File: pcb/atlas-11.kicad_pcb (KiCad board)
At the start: 2 copper layers, 115.2 x 61.7 mm, 37 parts, among them J1 USB, J2 DCJ-11 SBC Expansion Bus, J3 Micro_SD_Card_Det2, J4 DCJ-11 SBC Bus Probe Interface, SW1 SW_Push, SW2 SW_Push, U1 RP2350B-QFN80, U2 TPS22810DBVR, U4 NCP1117-3.3_SOT223, Y1 ABM8-272-T3

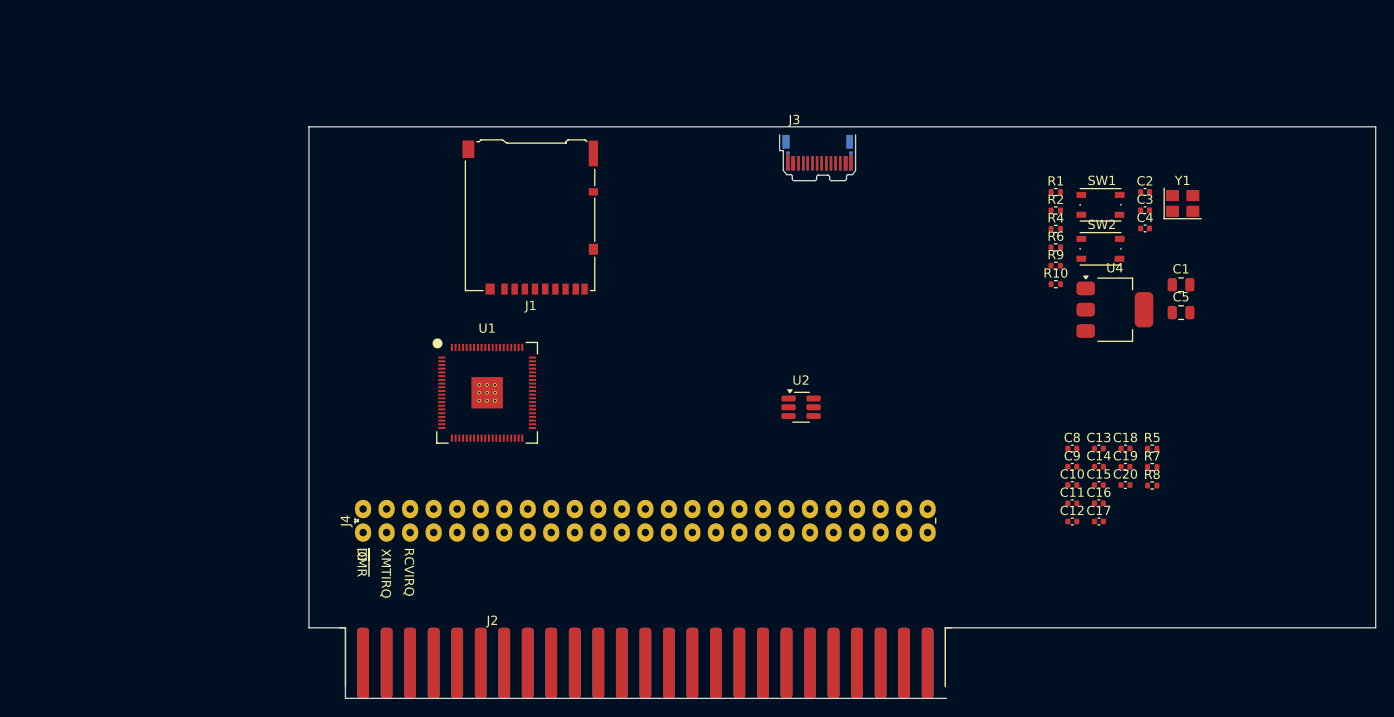
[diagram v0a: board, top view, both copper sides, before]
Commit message: pcb work
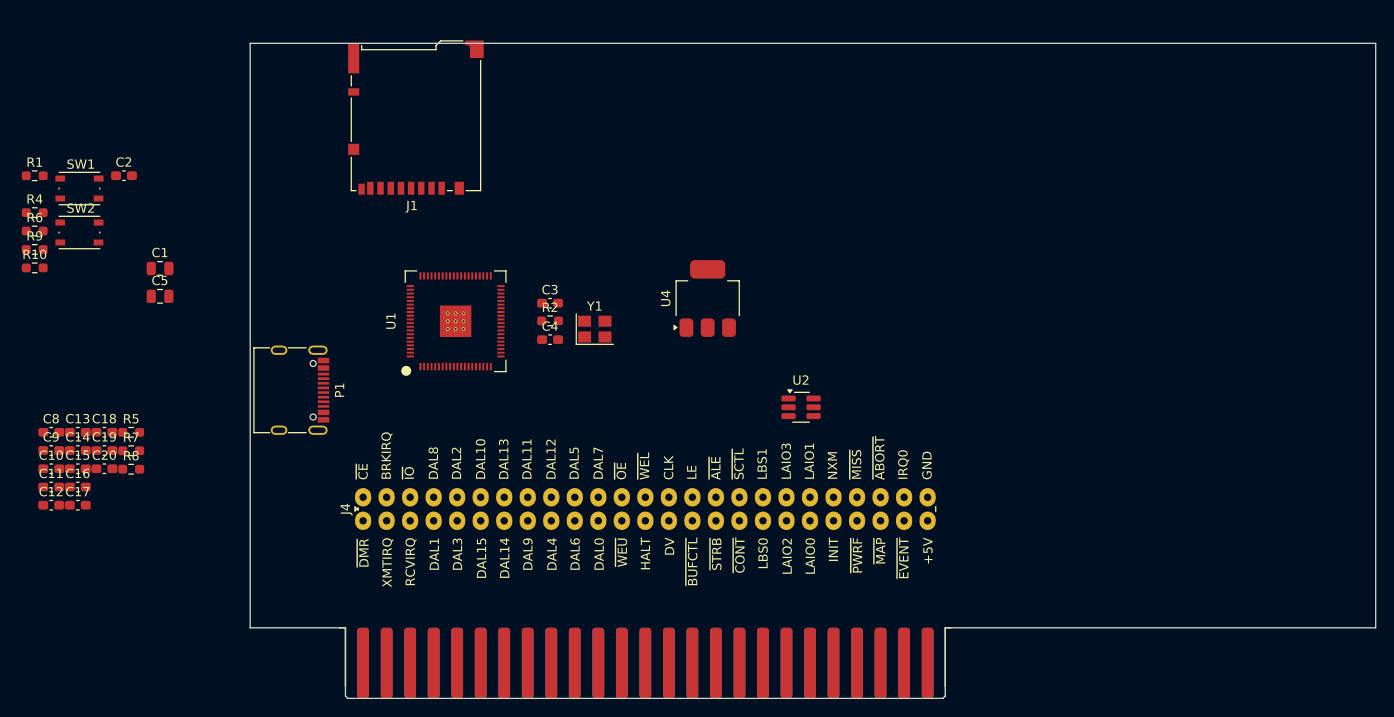
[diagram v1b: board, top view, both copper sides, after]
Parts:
- removed J3: Micro_SD_Card_Det2, Connector_USB:USB_C_Plug_JAE_DX07P024AJ1
- added P1: USB, Connector_USB:USB_C_Receptacle_G-Switch_GT-USB-7010ASV, F.Cu at (36.7, 83.1)
- C10, C11, C12, C13, C14, C15, C16, C17, C18, C19, C2, C20, C3, C4, C8, C9: footprint Capacitor_SMD:C_0402_1005Metric -> Capacitor_SMD:C_0603_1608Metric_Pad1.08x0.95mm_HandSolder
- J1: value USB -> Micro_SD_Card_Det1; footprint Connector_Card:microSD_HC_Hirose_DM3AT-SF-PEJM5 -> Connector_Card:microSD_HC_Hirose_DM3BT-DSF-PEJS
- R1, R10, R2, R4, R5, R6, R7, R8, R9: footprint Resistor_SMD:R_0402_1005Metric -> Resistor_SMD:R_0603_1608Metric_Pad0.98x0.95mm_HandSolder
- SW1: value SW_Push -> USB BOOT
- SW2: value SW_Push -> RUN
- moved C13 110.3 mm to (13.9, 87.6)
- moved C14 110.3 mm to (13.9, 89.6)
- moved C15 110.3 mm to (13.9, 91.5)
- moved C16 110.3 mm to (13.9, 93.5)
- moved C17 110.3 mm to (13.9, 95.5)
- moved C2 110.3 mm to (18.9, 59.9)
- moved R5 110.3 mm to (19.7, 87.6)
- moved R7 110.3 mm to (19.7, 89.6)
- moved R8 110.3 mm to (19.7, 91.6)
- moved C1 110.3 mm to (22.8, 69.9)
- moved C10 110.3 mm to (11.0, 91.5)
- moved C11 110.3 mm to (11.0, 93.5)
- moved C12 110.3 mm to (11.0, 95.5)
- moved C18 110.3 mm to (16.8, 87.6)
- moved C19 110.3 mm to (16.8, 89.6)
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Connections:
- net /~{USB_BOOT} renamed Net-(R6-Pad2)
- J1 pad 1: (no net) -> unconnected-(J1-DAT2-Pad1)
- J1 pad 10: (no net) -> unconnected-(J1-SHIELD-Pad10)
- J1 pad 2: (no net) -> SDCARD_CS
- J1 pad 3: (no net) -> SDCARD_MOSI
- J1 pad 4: (no net) -> +3V3
- J1 pad 5: (no net) -> SDCARD_CLK
- J1 pad 6: (no net) -> GND
- J1 pad 7: (no net) -> SDCARD_MISO
- J1 pad 8: (no net) -> unconnected-(J1-DAT1-Pad8)
- J1 pad 9: (no net) -> SDCARD_DET
- J2 pad 13: /HALT -> HALT
- J2 pad 15: /~{BUFCTL} -> ~{BUFCTL}
- J2 pad 17: /~{CONT} -> ~{CONT}
- J2 pad 21: /INIT -> INIT
- J2 pad 34: /~{SCTL} -> ~{SCTL}
- J2 pad 35: /~{ALE} -> ~{ALE}
- J2 pad 48: /~{IO} -> ~{IO}
- J4 pad 13: /HALT -> HALT
- J4 pad 15: /~{BUFCTL} -> ~{BUFCTL}
- J4 pad 17: /~{CONT} -> ~{CONT}
- J4 pad 21: /INIT -> INIT
- J4 pad 34: /~{SCTL} -> ~{SCTL}
- J4 pad 35: /~{ALE} -> ~{ALE}
- J4 pad 48: /~{IO} -> ~{IO}
- R4 pad 1: Net-(R4-Pad1) -> Net-(U1-RUN)
- R4 pad 2: GND -> Net-(R4-Pad2)
- SW2 pad 1: Net-(R4-Pad1) -> GND
- SW2 pad 2: Net-(U1-RUN) -> Net-(R4-Pad2)
- U1 pad 21: unconnected-(U1-GPIO21-Pad21) -> ~{BUFCTL}
- U1 pad 22: unconnected-(U1-GPIO22-Pad22) -> HALT
- U1 pad 23: unconnected-(U1-GPIO23-Pad23) -> ~{ALE}
- U1 pad 25: unconnected-(U1-GPIO24-Pad25) -> ~{SCTL}
- U1 pad 26: unconnected-(U1-GPIO25-Pad26) -> ~{CONT}
- U1 pad 27: unconnected-(U1-GPIO26-Pad27) -> INIT
- U1 pad 28: unconnected-(U1-GPIO27-Pad28) -> ~{IO}
- U1 pad 33: unconnected-(U1-SWCLK-Pad33) -> /SWCLK
- U1 pad 34: unconnected-(U1-SWDIO-Pad34) -> /SWDIO
- U1 pad 53: unconnected-(U1-GPIO42_ADC2-Pad53) -> SDCARD_DET
- U1 pad 54: unconnected-(U1-GPIO43_ADC3-Pad54) -> SDCARD_MOSI
- U1 pad 55: unconnected-(U1-GPIO44_ADC4-Pad55) -> SDCARD_MISO
- U1 pad 56: unconnected-(U1-GPIO45_ADC5-Pad56) -> SDCARD_CS
- U1 pad 57: unconnected-(U1-GPIO46_ADC6-Pad57) -> SDCARD_CLK
- U1 pad 77: unconnected-(U1-GPIO0-Pad77) -> UART0_TX
- U1 pad 78: unconnected-(U1-GPIO1-Pad78) -> UART0_RX
- U1 pad 81: unconnected-(U1-GND-Pad81) -> GND
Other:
- board size 115.2 x 61.7 mm -> 121.5 x 70.7 mm

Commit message: pcb work
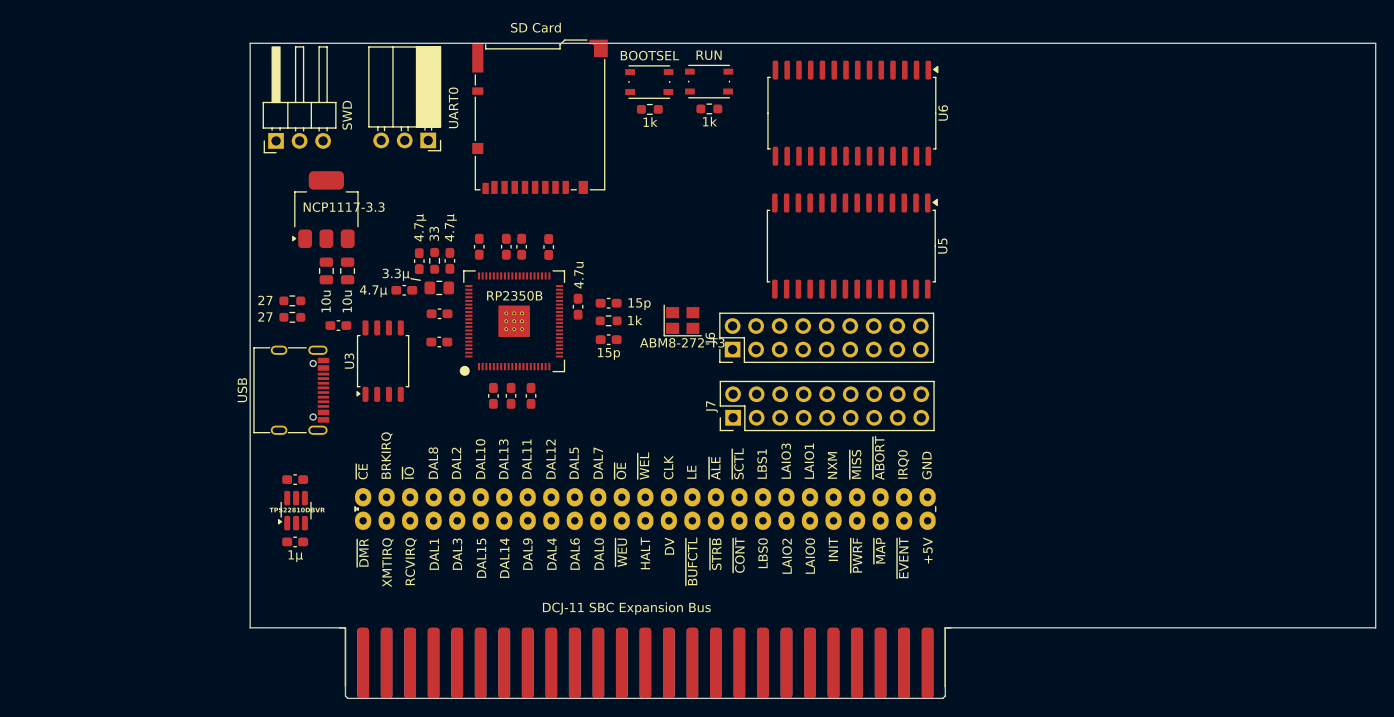
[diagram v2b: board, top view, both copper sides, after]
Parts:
- removed R1, R9: DNF, Resistor_SMD:R_0603_1608Metric_Pad0.98x0.95mm_HandSolder
- removed R10: 0, Resistor_SMD:R_0603_1608Metric_Pad0.98x0.95mm_HandSolder
- added C21: 4.7µ, Capacitor_SMD:C_0603_1608Metric_Pad1.08x0.95mm_HandSolder, F.Cu at (50.8, 69.1)
- added C7: 4.7µ, Capacitor_SMD:C_0603_1608Metric_Pad1.08x0.95mm_HandSolder, F.Cu at (49.1, 72.3)
- added J3: SWD, Connector_PinHeader_2.54mm:PinHeader_1x03_P2.54mm_Horizontal, F.Cu at (35.3, 56.1)
- added J5: UART0, Connector_PinSocket_2.54mm:PinSocket_1x03_P2.54mm_Horizontal, F.Cu at (51.7, 56.1)
- added J6: User Port, Connector_PinHeader_2.54mm:PinHeader_2x09_P2.54mm_Vertical, F.Cu at (84.6, 78.7)
- added J7: Pico Bits, Connector_PinHeader_2.54mm:PinHeader_2x09_P2.54mm_Vertical, F.Cu at (84.7, 86.0)
- added L1: 3.3µ, Inductor_SMD:L_0805_2012Metric_Pad1.15x1.40mm_HandSolder, F.Cu at (52.9, 72.0)
- added U3: W25Q128JVS, Package_SO:SOIC-8_5.3x5.3mm_P1.27mm, F.Cu at (46.9, 79.9)
- added U5: MCP23017, Package_SO:SOIC-28W_7.5x17.9mm_P1.27mm, F.Cu at (97.4, 67.5)
- added U6: MCP23017_SO, Package_SO:SOIC-28W_7.5x17.9mm_P1.27mm, F.Cu at (97.5, 53.1)
- C9: value 4.7u -> 4.7µ
- J1: value Micro_SD_Card_Det1 -> SD Card
- SW1: value USB BOOT -> BOOTSEL
- U1: value RP2350B-QFN80 -> RP2350B
- U4: value NCP1117-3.3_SOT223 -> NCP1117-3.3
- moved R4 73.7 mm to (82.1, 52.7), turned to 180 degrees
- moved SW2 69.9 mm to (82.1, 49.7)
- moved R6 67.7 mm to (75.7, 52.7), turned to 180 degrees
- moved SW1 62.6 mm to (75.6, 49.8)
- moved C10 59.5 mm to (67.9, 74.0), turned to 90 degrees
- moved C17 58.0 mm to (64.7, 67.6), turned to 90 degrees
- moved C12 58.0 mm to (61.8, 67.6), turned to 90 degrees
- moved U2 55.7 mm to (37.5, 96.1), turned to 90 degrees
- moved C8 53.1 mm to (60.2, 67.6), turned to 90 degrees
- moved C11 50.6 mm to (60.7, 83.7), turned to -90 degrees
- moved C16 50.5 mm to (57.3, 67.6), turned to 90 degrees
- moved C9 47.7 mm to (54.1, 69.1), turned to 90 degrees
- moved C18 46.2 mm to (62.8, 83.7), turned to -90 degrees
- moved C13 45.0 mm to (58.8, 83.7), turned to -90 degrees
- moved C15 42.5 mm to (53.0, 74.8), turned to 180 degrees
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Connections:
- U1 pad 1: unconnected-(U1-GPIO4-Pad1) -> LED1
- U1 pad 36: unconnected-(U1-GPIO28-Pad36) -> GPIO28
- U1 pad 37: unconnected-(U1-GPIO29-Pad37) -> GPIO29
- U1 pad 38: unconnected-(U1-GPIO30-Pad38) -> GPIO30
- U1 pad 39: unconnected-(U1-GPIO31-Pad39) -> GPIO31
- U1 pad 40: unconnected-(U1-GPIO32-Pad40) -> GPIO32
- U1 pad 42: unconnected-(U1-GPIO33-Pad42) -> GPIO33
- U1 pad 43: unconnected-(U1-GPIO34-Pad43) -> GPIO34
- U1 pad 44: unconnected-(U1-GPIO35-Pad44) -> GPIO35
- U1 pad 45: unconnected-(U1-GPIO36-Pad45) -> SINTA
- U1 pad 46: unconnected-(U1-GPIO37-Pad46) -> SINTB
- U1 pad 47: unconnected-(U1-GPIO38-Pad47) -> UINTA
- U1 pad 48: unconnected-(U1-GPIO39-Pad48) -> UINTB
- U1 pad 49: unconnected-(U1-GPIO40_ADC0-Pad49) -> SDA
- U1 pad 52: unconnected-(U1-GPIO41_ADC1-Pad52) -> SCL
- U1 pad 58: unconnected-(U1-GPIO47_ADC7-Pad58) -> GPIO47
- U1 pad 80: unconnected-(U1-GPIO3-Pad80) -> LED0
